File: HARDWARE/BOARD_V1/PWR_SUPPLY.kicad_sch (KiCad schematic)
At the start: 28 parts, among them IC1 AP3441LSHE-7B, IC2 LDLN025M33R, IC3 LDLN025M33R, IC4 LDLN025M33R, IC5 AP3441LSHE-7B

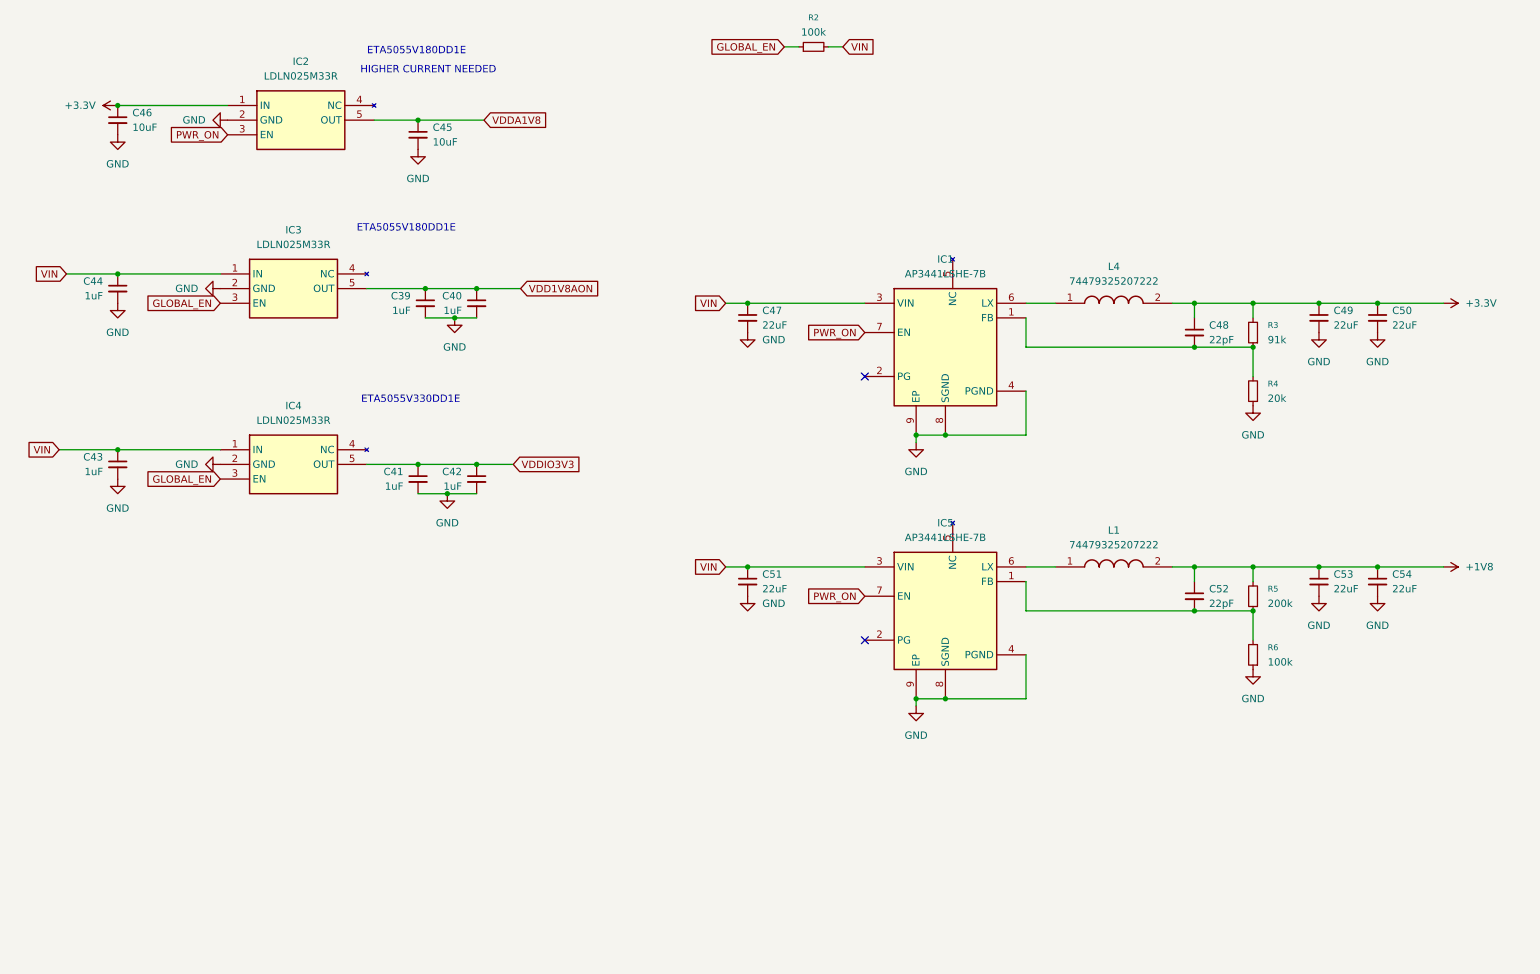
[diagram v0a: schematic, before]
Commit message: up
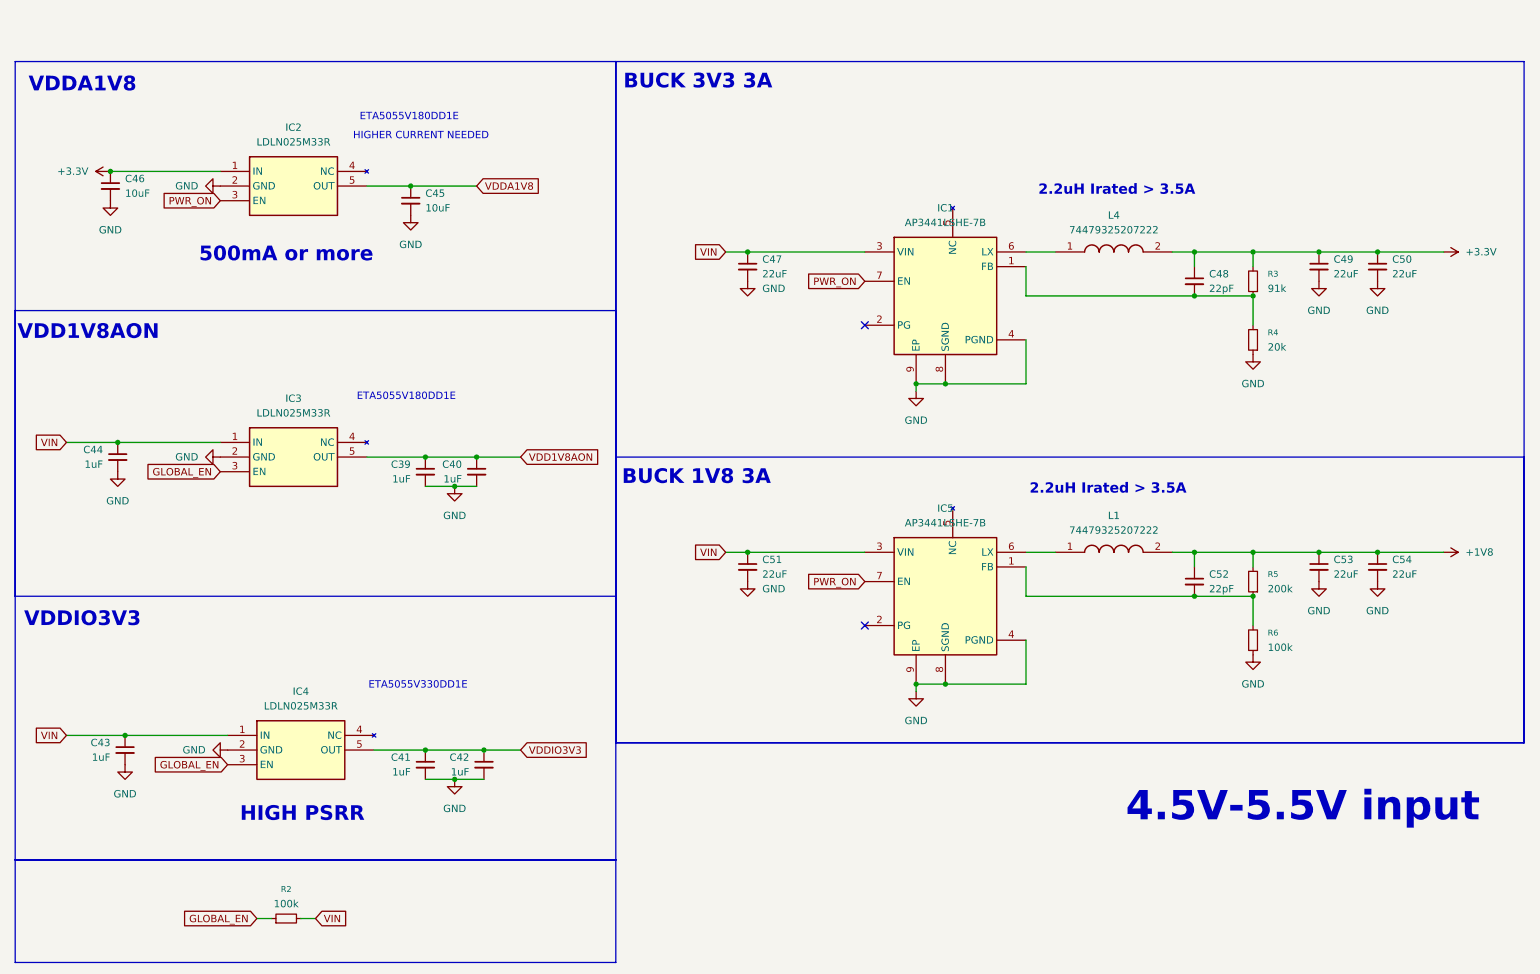
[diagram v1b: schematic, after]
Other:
- note added: "2.2uH Irated > 3.5A"
- note added: "4.5V-5.5V input"
- note added: "500mA or more"
- note added: "BUCK 1V8 3A"
- note added: "BUCK 3V3 3A"
- note added: "HIGH PSRR"
- note added: "VDD1V8AON"
- note added: "VDDA1V8"
- note added: "VDDIO3V3"
- moved on the sheet: C39, C40, C41, C42, C43, C44, C45, C46, C47, C48, C49, C50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
